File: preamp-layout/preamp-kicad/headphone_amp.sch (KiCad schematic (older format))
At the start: 22 parts, among them J32 Conn_01x03_Male, J35 Conn_01x05_Male, J58 Conn_01x03_Male, J61 Conn_01x03_Male, J62 Conn_01x03_Male, U19 TPA6120

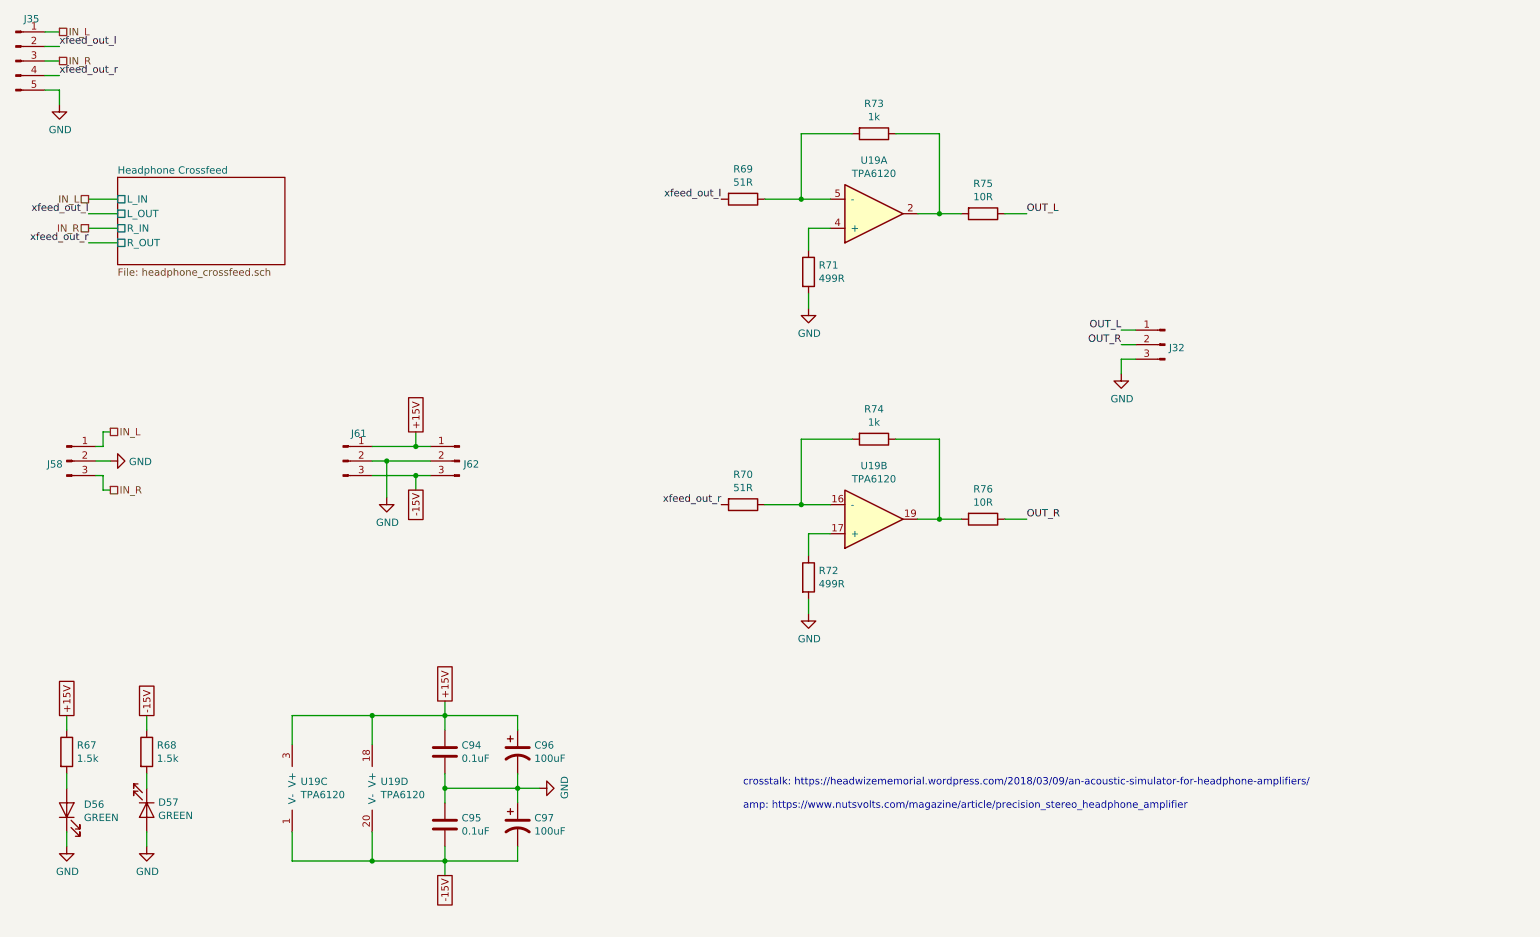
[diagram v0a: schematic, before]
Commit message: PCB layout
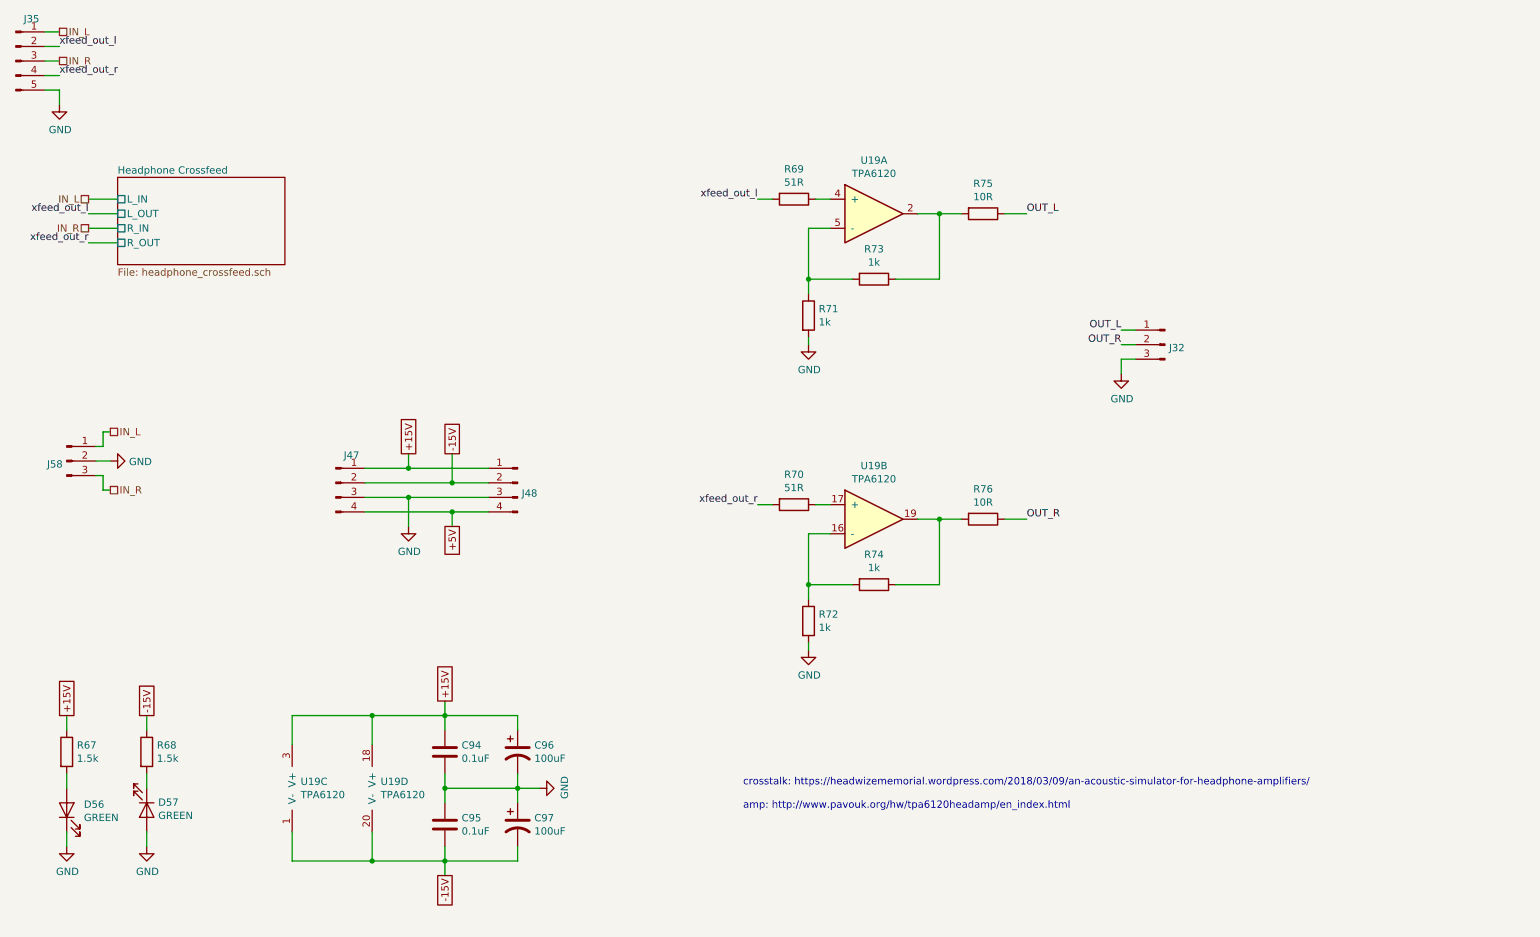
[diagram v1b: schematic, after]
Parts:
- removed J61, J62: Conn_01x03_Male, Connector_JST:JST_EH_S3B-EH_1x03_P2.50mm_Horizontal, symbol Connector:Conn_01x03_Male
- added J47, J48: Conn_01x04_Male, Connector_JST:JST_EH_S4B-EH_1x04_P2.50mm_Horizontal, symbol Connector:Conn_01x04_Male
- R71, R72: value 499R -> 1k
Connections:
- net +15V: now also J47.1 (Pin_1), J48.1 (Pin_1)
- net -15V: now also J47.2 (Pin_2), J48.2 (Pin_2)
- net GND: now also J47.3 (Pin_3), J48.3 (Pin_3)
- net at U19.4 (+): now also R69.1; no longer R71.1
- net at R73.2, U19.5 (-): now also R71.1; no longer R69.1
- net at R74.2, U19.16 (-): now also R72.1; no longer R70.1
- net at U19.17 (+): now also R70.1; no longer R72.1
- new net +5V: J47.4 (Pin_4), J48.4 (Pin_4)
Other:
- note added: "crosstalk: https://headwizememorial.wordpress.com/2018/03/09/an-acoustic-simulator-for-headphone-amplifiers/\n\namp: http://www.pavouk.org/hw/tpa6120headamp/en_index.html"
- note removed: "crosstalk: https://headwizememorial.wordpress.com/2018/03/09/an-acoustic-simulator-for-headphone-amplifiers/\n\namp: https://www.nutsvolts.com/magazine/article/precision_stereo_headphone_amplifier"
- moved on the sheet: R69, R70, R71, R72, R73, R74
